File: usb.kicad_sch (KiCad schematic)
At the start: 4 parts, among them J2 USB_C_Receptacle_USB2.0_14P, U4 TPD2EUSB30

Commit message: design pcb and place components
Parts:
- R13, R14: footprint Resistor_SMD:R_0805_2012Metric -> Resistor_SMD:R_0402_1005Metric; LCSC C27834 -> (none)
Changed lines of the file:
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@@
 			)
 		)
-		(property "Footprint" "Resistor_SMD:R_0805_2012Metric"
+		(property "Footprint" "Resistor_SMD:R_0402_1005Metric"
 			(at 146.812 116.84 90)
 			(hide yes)
@@
 		)
 		(property "Description" "Resistor"
-			(at 148.59 116.84 0)
-			(hide yes)
-			(show_name no)
-			(do_not_autoplace no)
-			(effects
-				(font
-					(size 1.27 1.27)
-				)
-			)
-		)
-		(property "LCSC" "C27834"
 			(at 148.59 116.84 0)
 			(hide yes)
@@
 			)
 		)
-		(property "Footprint" "Resistor_SMD:R_0805_2012Metric"
+		(property "Footprint" "Resistor_SMD:R_0402_1005Metric"
 			(at 143.002 116.84 90)
 			(hide yes)
@@
 			(at 144.78 116.84 0)
 			(hide yes)
-			(show_name no)
-			(do_not_autoplace no)
-			(effects
-				(font
-					(size 1.27 1.27)
-				)
-			)
-		)
-		(property "LCSC" "C27834"
-			(at 144.78 116.84 0)
-			(hide yes)

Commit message: tentative automatic population
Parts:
- J2: MPN (none) -> GT-USB-7010ASV; Manufacturer (none) -> G-Switch
- R13, R14: LCSC (none) -> C25905; MPN (none) -> 0402WGF5101TCE; Manufacturer (none) -> UNI-ROYAL
- U4: LCSC C97502 -> C94934; MPN (none) -> TPD2EUSB30ADRTR; Manufacturer (none) -> TI
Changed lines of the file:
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@@
+			)
+		)
+		(property "Manufacturer" "G-Switch" (at 0 0 0)
+			(effects
+				(font
+					(size 1.27 1.27)
+				)
+				(hide yes)
+			)
+		)
+		(property "MPN" "GT-USB-7010ASV" (at 0 0 0)
+			(effects
+				(font
+					(size 1.27 1.27)
+				)
+				(hide yes)
 			)
 		)
@@
 			)
 		)
-		(property "Datasheet" ""
+		(property "Datasheet" "https://datasheet.lcsc.com/datasheet/pdf/0a975aaa49b7c97f38a963127be4a823.pdf?productCode=C25905"
 			(at 148.59 116.84 0)
 			(hide yes)
@@
 					(size 1.27 1.27)
 				)
+			)
+		)
+		(property "Manufacturer" "UNI-ROYAL" (at 0 0 0)
+			(effects
+				(font
+					(size 1.27 1.27)
+				)
+				(hide yes)
+			)
+		)
+		(property "MPN" "0402WGF5101TCE" (at 0 0 0)
+			(effects
+				(font
+					(size 1.27 1.27)
+				)
+				(hide yes)
+			)
+		)
+		(property "LCSC" "C25905" (at 0 0 0)
+			(effects
+				(font
+					(size 1.27 1.27)
+				)
+				(hide yes)
 			)
 		)
@@
 			)
 		)
-		(property "Datasheet" ""
+		(property "Datasheet" "https://datasheet.lcsc.com/datasheet/pdf/0a975aaa49b7c97f38a963127be4a823.pdf?productCode=C25905"
 			(at 144.78 116.84 0)
 			(hide yes)
@@
 					(size 1.27 1.27)
 				)
+			)
+		)
+		(property "Manufacturer" "UNI-ROYAL" (at 0 0 0)
+			(effects
+				(font
+					(size 1.27 1.27)
+				)
+				(hide yes)
+			)
+		)
+		(property "MPN" "0402WGF5101TCE" (at 0 0 0)
+			(effects
+				(font
+					(size 1.27 1.27)
+				)
+				(hide yes)
+			)
+		)
+		(property "LCSC" "C25905" (at 0 0 0)
+			(effects
+				(font
+					(size 1.27 1.27)
+				)
+				(hide yes)
 			)
 		)
@@
 			)
 		)
-		(property "LCSC" "C97502"
+		(property "LCSC" "C94934"
 			(at 162.56 109.22 0)
 			(hide yes)
@@
 			)
 		)
+		(property "Manufacturer" "TI" (at 0 0 0)
+			(effects
+				(font
+					(size 1.27 1.27)
+				)
+				(hide yes)
+			)
+		)
+		(property "MPN" "TPD2EUSB30ADRTR" (at 0 0 0)
+			(effects
+				(font
+					(size 1.27 1.27)
+				)
+				(hide yes)
+			)
+		)

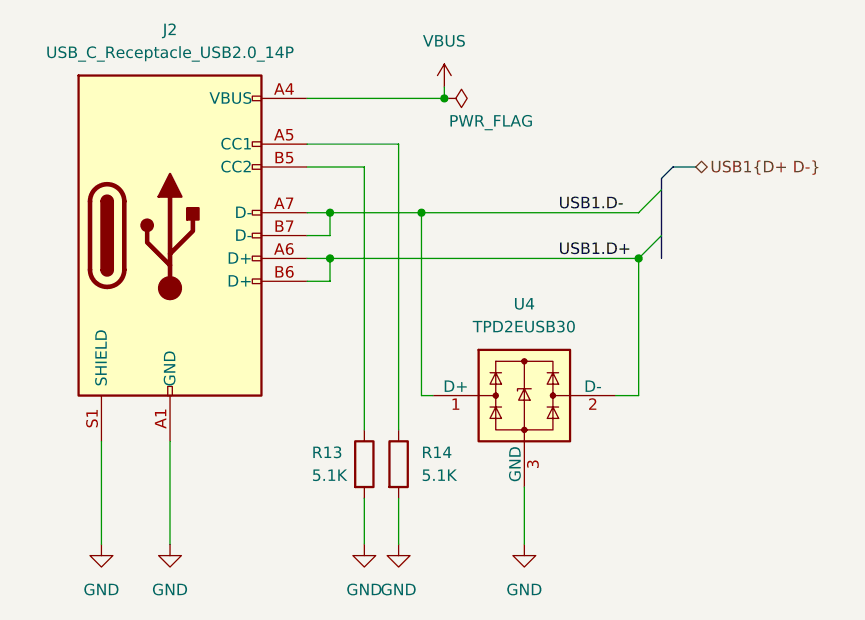
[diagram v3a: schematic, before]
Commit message: finalized component selection
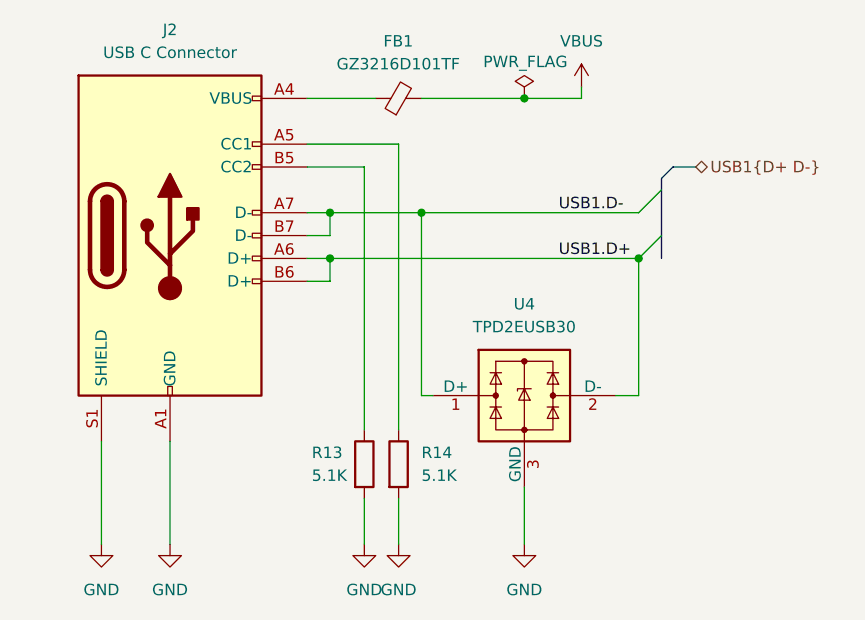
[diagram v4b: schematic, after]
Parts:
- added FB1: GZ3216D101TF, Inductor_SMD:L_1206_3216Metric, symbol Device:FerriteBead_Small
- J2: value USB_C_Receptacle_USB2.0_14P -> USB C Connector
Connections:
- net VBUS: now also FB1.2; no longer J2.A4 (VBUS), J2.A9 (VBUS), J2.B4 (VBUS), J2.B9 (VBUS)
- new net: FB1.1, J2.A4 (VBUS), J2.A9 (VBUS), J2.B4 (VBUS), J2.B9 (VBUS)
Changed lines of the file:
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@@
+	)
+	(junction
+		(at 162.56 76.2)
+		(diameter 0)
+		(color 0 0 0 0)
 	)
 	(junction
@@
 	)
 	(junction
-		(at 153.67 76.2)
-		(diameter 0)
-		(color 0 0 0 0)
-	)
-	(junction
 		(at 175.26 93.98)
 		(diameter 0)
@@
 	(wire
 		(pts
+			(xy 162.56 76.2) (xy 168.91 76.2)
+		)
+		(stroke
+			(width 0)
+			(type default)
+		)
+	)
+	(wire
+		(pts
 			(xy 138.43 83.82) (xy 144.78 83.82)
 		)
@@
 	(wire
 		(pts
+			(xy 138.43 76.2) (xy 146.05 76.2)
+		)
+		(stroke
+			(width 0)
+			(type default)
+		)
+	)
+	(wire
+		(pts
 			(xy 144.78 120.65) (xy 144.78 125.73)
 		)
@@
 	(wire
 		(pts
-			(xy 138.43 76.2) (xy 153.67 76.2)
+			(xy 151.13 76.2) (xy 162.56 76.2)
 		)
 		(stroke
@@
 	(wire
 		(pts
-			(xy 153.67 76.2) (xy 153.67 74.93)
+			(xy 168.91 76.2) (xy 168.91 74.93)
 		)
 		(stroke
@@
 			)
 		)
-		(property "Value" "USB_C_Receptacle_USB2.0_14P"
+		(property "Value" "USB C Connector"
 			(at 123.19 71.12 0)
 			(show_name no)
@@
 	(symbol
 		(lib_id "power:VBUS")
-		(at 153.67 74.93 0)
+		(at 168.91 74.93 0)
 		(unit 1)
 		(body_style 1)
@@
 		(fields_autoplaced yes)
 		(property "Reference" "#PWR047"
-			(at 153.67 78.74 0)
+			(at 168.91 78.74 0)
 			(hide yes)
 			(show_name no)
@@
 		)
 		(property "Value" "VBUS"
-			(at 153.67 69.85 0)
+			(at 168.91 69.85 0)
 			(show_name no)
 			(do_not_autoplace no)
@@
 		)
 		(property "Footprint" ""
-			(at 153.67 74.93 0)
+			(at 168.91 74.93 0)
 			(hide yes)
 			(show_name no)
@@
 		)
 		(property "Datasheet" ""
-			(at 153.67 74.93 0)
+			(at 168.91 74.93 0)
 			(hide yes)
 			(show_name no)
@@
 		)
 		(property "Description" "Power symbol creates a global label with name \"VBUS\""
-			(at 153.67 74.93 0)
+			(at 168.91 74.93 0)
 			(hide yes)
 			(show_name no)
@@
 	)
 	(symbol
+		(lib_id "Device:FerriteBead_Small")
+		(at 148.59 76.2 90)
+		(unit 1)
+		(body_style 1)
+		(exclude_from_sim no)
+		(in_bom yes)
+		(on_board yes)
+		(in_pos_files yes)
+		(dnp no)
+		(fields_autoplaced yes)
+		(property "Reference" "FB1"
+			(at 148.5519 69.85 90)
+			(show_name no)
+			(do_not_autoplace no)
+			(effects
+				(font
+					(size 1.27 1.27)
+				)
+			)
+		)
+		(property "Value" "GZ3216D101TF"
+			(at 148.5519 72.39 90)
+			(show_name no)
+			(do_not_autoplace no)
+			(effects
+				(font
+					(size 1.27 1.27)
+				)
+			)
+		)
+		(property "Footprint" "Inductor_SMD:L_1206_3216Metric"
+			(at 148.59 77.978 90)
+			(hide yes)
+			(show_name no)
+			(do_not_autoplace no)
+			(effects
+				(font
+					(size 1.27 1.27)
+				)
+			)
+		)
+		(property "Datasheet" ""
+			(at 148.59 76.2 0)
+			(hide yes)
+			(show_name no)
+			(do_not_autoplace no)
+			(effects
+				(font
+					(size 1.27 1.27)
+				)
+			)
+		)
+		(property "Description" "Ferrite bead, small symbol"
+			(at 148.59 76.2 0)
+			(hide yes)
+			(show_name no)
+			(do_not_autoplace no)
+			(effects
+				(font
+					(size 1.27 1.27)
+				)
+			)
+		)
+		(property "LCSC" "C369799"
+			(at 148.59 76.2 90)
+			(hide yes)
+			(show_name no)
+			(do_not_autoplace no)
+			(effects
+				(font
+					(size 1.27 1.27)
+				)
+			)
+		)
+		(pin "2"
+		)
+		(pin "1"
+		)
+		(instances
+			(project "rover-circuit"
+				(path "/0461baee-3b25-4e1a-a5c1-d76b4b99c66c/5070e061-e1bc-4e4d-b169-49ea5dd67ecf"
+					(reference "FB1")
+					(unit 1)
+				)
+			)
+		)
+	)
+	(symbol
 		(lib_id "power:GND")
 		(at 123.19 125.73 0)
@@
 	(symbol
 		(lib_id "power:PWR_FLAG")
-		(at 153.67 76.2 270)
+		(at 162.56 76.2 0)
 		(unit 1)
 		(body_style 1)
@@
 		(dnp no)
 		(property "Reference" "#FLG07"
-			(at 155.575 76.2 0)
+			(at 162.56 74.295 0)
 			(hide yes)
 			(show_name no)
@@
 		)
 		(property "Value" "PWR_FLAG"
-			(at 154.178 78.74 90)
+			(at 157.988 72.136 0)
 			(show_name no)
 			(do_not_autoplace no)
@@
 		)
 		(property "Footprint" ""
-			(at 153.67 76.2 0)
+			(at 162.56 76.2 0)
 			(hide yes)
 			(show_name no)
@@
 		)
 		(property "Datasheet" ""
-			(at 153.67 76.2 0)
+			(at 162.56 76.2 0)
 			(hide yes)
 			(show_name no)
@@
 		)
 		(property "Description" "Special symbol for telling ERC where power comes from"
-			(at 153.67 76.2 0)
-			(hide yes)
-			(show_name no)
+			(at 162.56 76.2 0)
+			(hide yes)
+			(show_name no)

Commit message: add MPS entries
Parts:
- FB1: MPN (none) -> BLM31PG500SN1L; Manufacturer (none) -> Murata
- R13, R14: MPN 0402WGF5101TCE -> GPN; Manufacturer UNI-ROYAL -> Generic
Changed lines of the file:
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@@
 			)
 		)
-		(property "Manufacturer" "UNI-ROYAL"
+		(property "Manufacturer" "Generic"
 			(at 0 0 0)
 			(hide yes)
@@
 			)
 		)
-		(property "MPN" "0402WGF5101TCE"
+		(property "MPN" "GPN"
 			(at 0 0 0)
 			(hide yes)
@@
 			)
 		)
+		(property "Manufacturer" "Murata" (at 0 0 0)
+			(effects
+				(font
+					(size 1.27 1.27)
+				)
+				(hide yes)
+			)
+		)
+		(property "MPN" "BLM31PG500SN1L" (at 0 0 0)
+			(effects
+				(font
+					(size 1.27 1.27)
+				)
+				(hide yes)
+			)
+		)
 		(pin "2"
 		)
@@
 			)
 		)
-		(property "Manufacturer" "UNI-ROYAL"
+		(property "Manufacturer" "Generic"
 			(at 0 0 0)
 			(hide yes)
@@
 			)
 		)
-		(property "MPN" "0402WGF5101TCE"
+		(property "MPN" "GPN"
 			(at 0 0 0)
 			(hide yes)

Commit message: update MPN codes
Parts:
- R13, R14: MPN GPN -> GPR040251
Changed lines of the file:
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@@
 			)
 		)
-		(property "MPN" "GPN"
+		(property "MPN" "GPR040251"
 			(at 0 0 0)
 			(hide yes)
@@
 			)
 		)
-		(property "Manufacturer" "Murata" (at 0 0 0)
-			(effects
-				(font
-					(size 1.27 1.27)
-				)
-				(hide yes)
-			)
-		)
-		(property "MPN" "BLM31PG500SN1L" (at 0 0 0)
-			(effects
-				(font
-					(size 1.27 1.27)
-				)
-				(hide yes)
+		(property "Manufacturer" "Murata"
+			(at 0 0 0)
+			(hide yes)
+			(show_name no)
+			(do_not_autoplace no)
+			(effects
+				(font
+					(size 1.27 1.27)
+				)
+			)
+		)
+		(property "MPN" "BLM31PG500SN1L"
+			(at 0 0 0)
+			(hide yes)
+			(show_name no)
+			(do_not_autoplace no)
+			(effects
+				(font
+					(size 1.27 1.27)
+				)
 			)
 		)
@@
 			)
 		)
-		(property "MPN" "GPN"
-			(at 0 0 0)
-			(hide yes)
+		(property "MPN" "GPR040251"
+			(at 0 0 0)
+			(hide yes)
